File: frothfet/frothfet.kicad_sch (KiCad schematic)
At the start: 8 parts, among them U1 ESP32-S3-DEVKITC

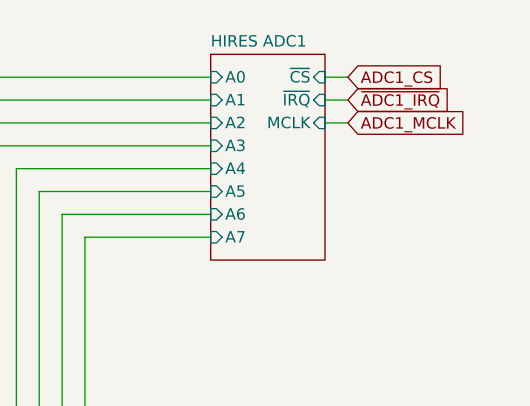
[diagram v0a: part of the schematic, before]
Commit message: updates
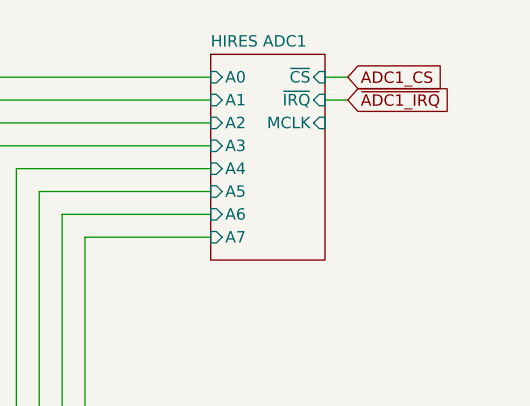
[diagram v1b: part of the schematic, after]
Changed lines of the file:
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@@
-	(wire
-		(pts
-			(xy 262.89 48.26) (xy 260.35 48.26)
-		)
-		(stroke
-			(width 0)
-			(type default)
-		)
-	)
 	(wire
 		(pts
@@
 			(effects
 				(font
-					(size 1.27 1.27)
-				)
-				(justify left)
-				(hide yes)
-			)
-		)
-	)
-	(global_label "ADC1_MCLK"
-		(shape input)
-		(at 262.89 48.26 0)
-		(fields_autoplaced yes)
-		(effects
-			(font
-				(size 1.27 1.27)
-			)
-			(justify left)
-		)
-		(property "Intersheetrefs" "${INTERSHEET_REFS}"
-			(at 276.7004 48.26 0)
-			(effects
-				(font

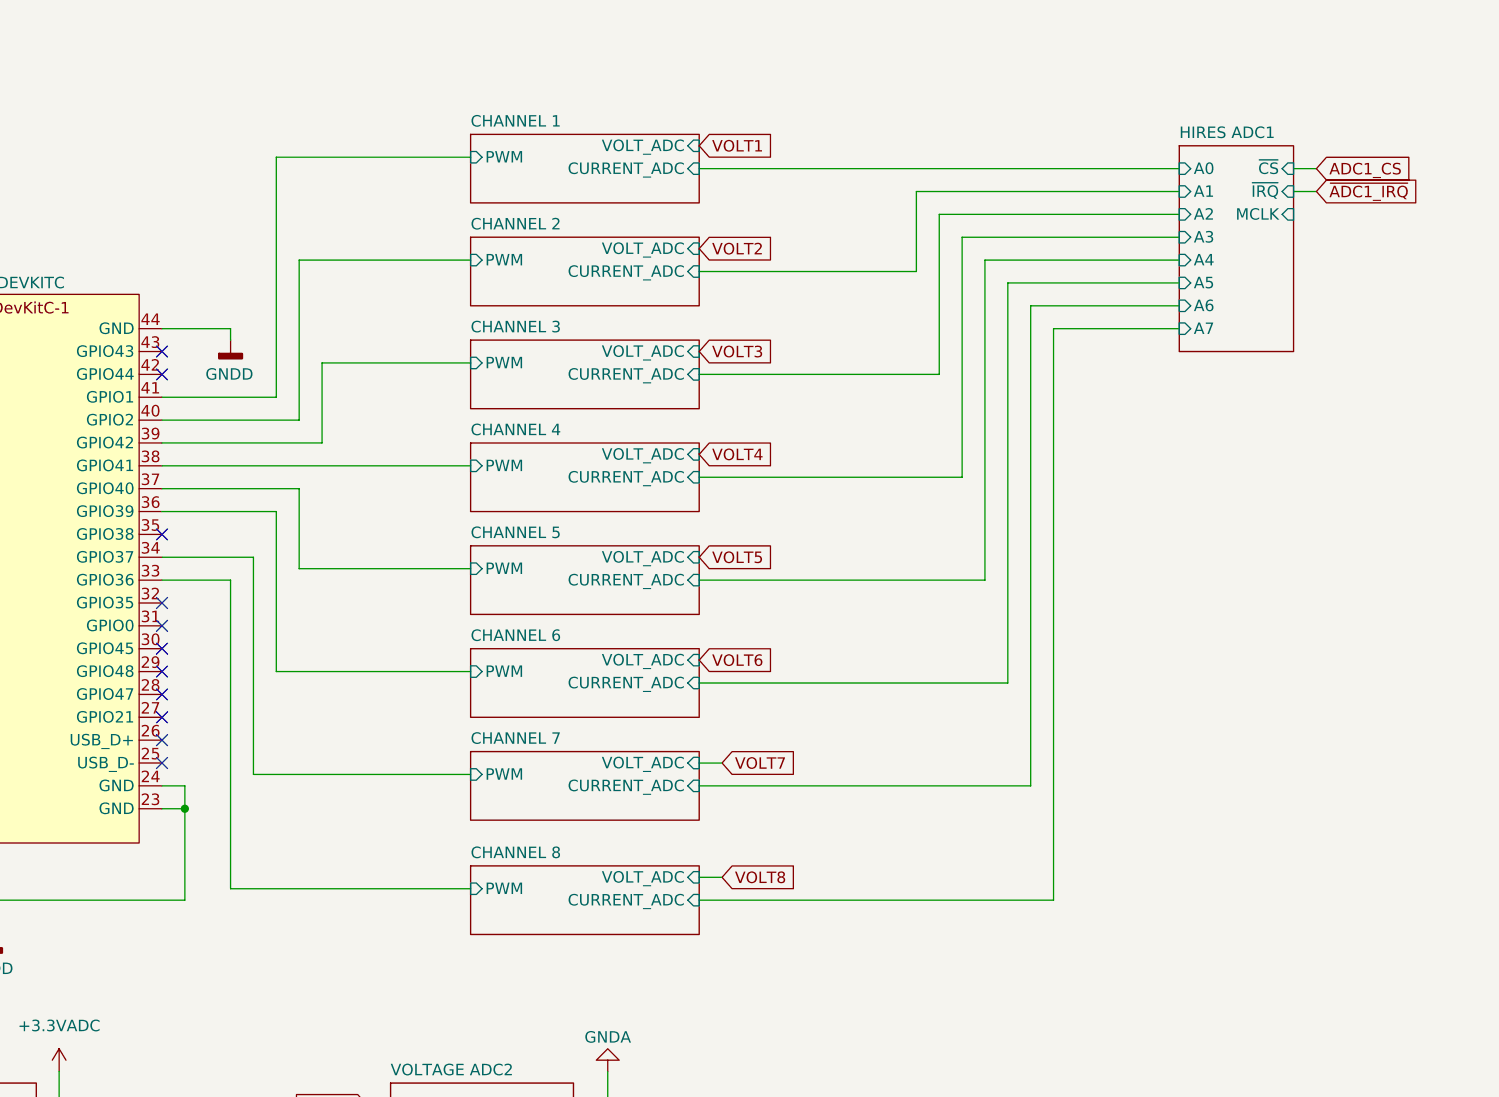
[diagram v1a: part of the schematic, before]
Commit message: rev e channel changes.
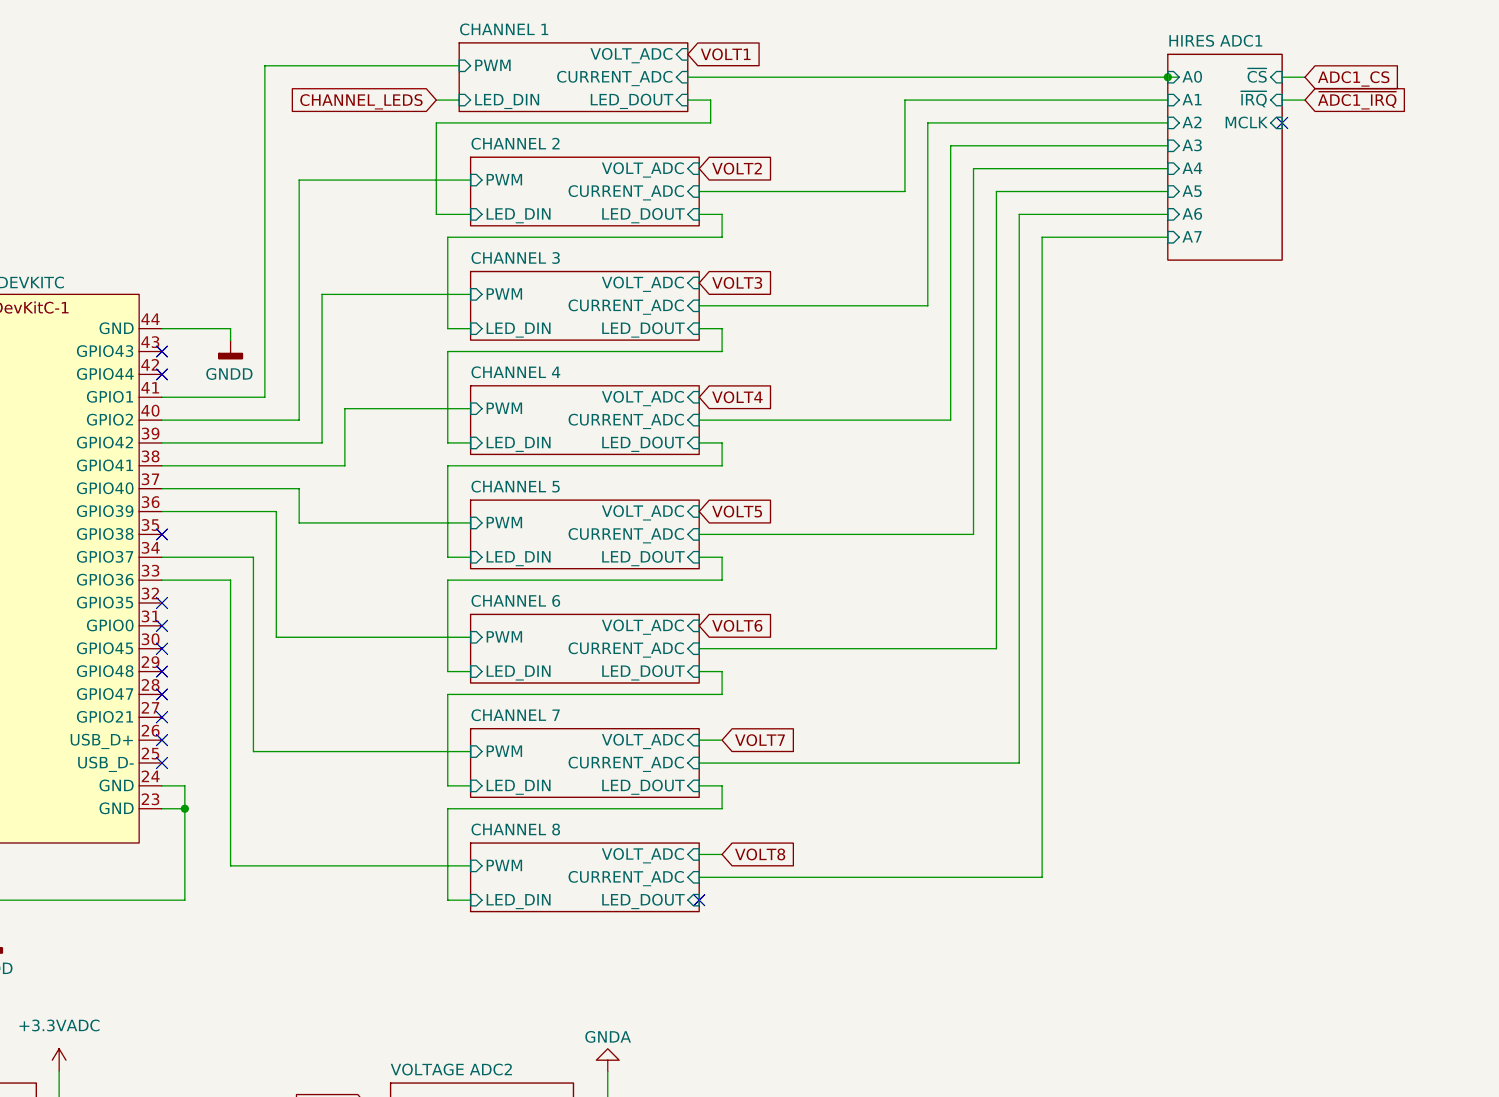
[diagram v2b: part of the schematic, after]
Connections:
- no-connect marks 16 -> 18
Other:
- sheet CHANNEL 1 ports: added LED_DIN, LED_DOUT; removed none
- sheet CHANNEL 2 ports: added LED_DIN, LED_DOUT; removed none
- sheet CHANNEL 3 ports: added LED_DIN, LED_DOUT; removed none
- sheet CHANNEL 4 ports: added LED_DIN, LED_DOUT; removed none
- sheet CHANNEL 5 ports: added LED_DIN, LED_DOUT; removed none
- sheet CHANNEL 6 ports: added LED_DIN, LED_DOUT; removed none
- sheet CHANNEL 7 ports: added LED_DIN, LED_DOUT; removed none
- sheet CHANNEL 8 ports: added LED_DIN, LED_DOUT; removed none
